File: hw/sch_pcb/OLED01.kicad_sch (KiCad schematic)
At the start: 59 parts, among them J1 HEADER_2x03_PARALLEL, J2 HEADER_2x03_PARALLEL, J3 HEADER_2x01_PARALLEL, J4 HEADER_2x03_PARALLEL, J5 HEADER_1x03, J6 HEADER_2x05_PARALLEL, Q1 BC817-25, Q2 BC817-25, Q3 BC817-25, U1 TLV840, U2 MIC5504-2.5YM5, U3 MAX5026, U5 PCA9306DP

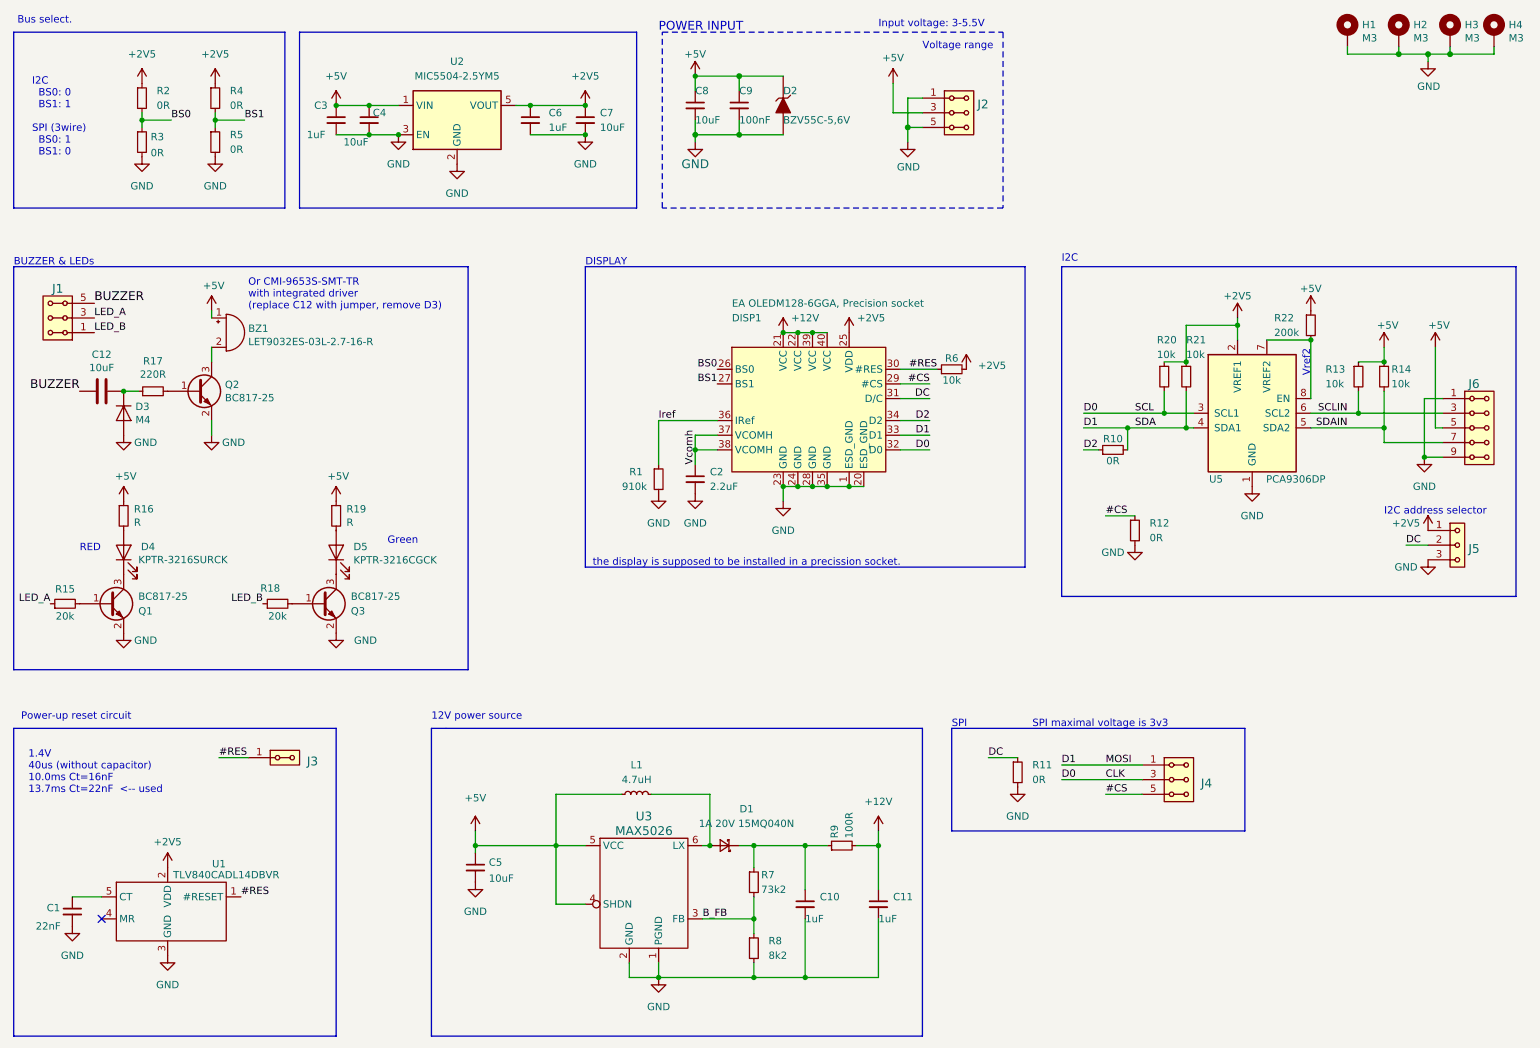
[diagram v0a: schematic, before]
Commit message: solve DRC
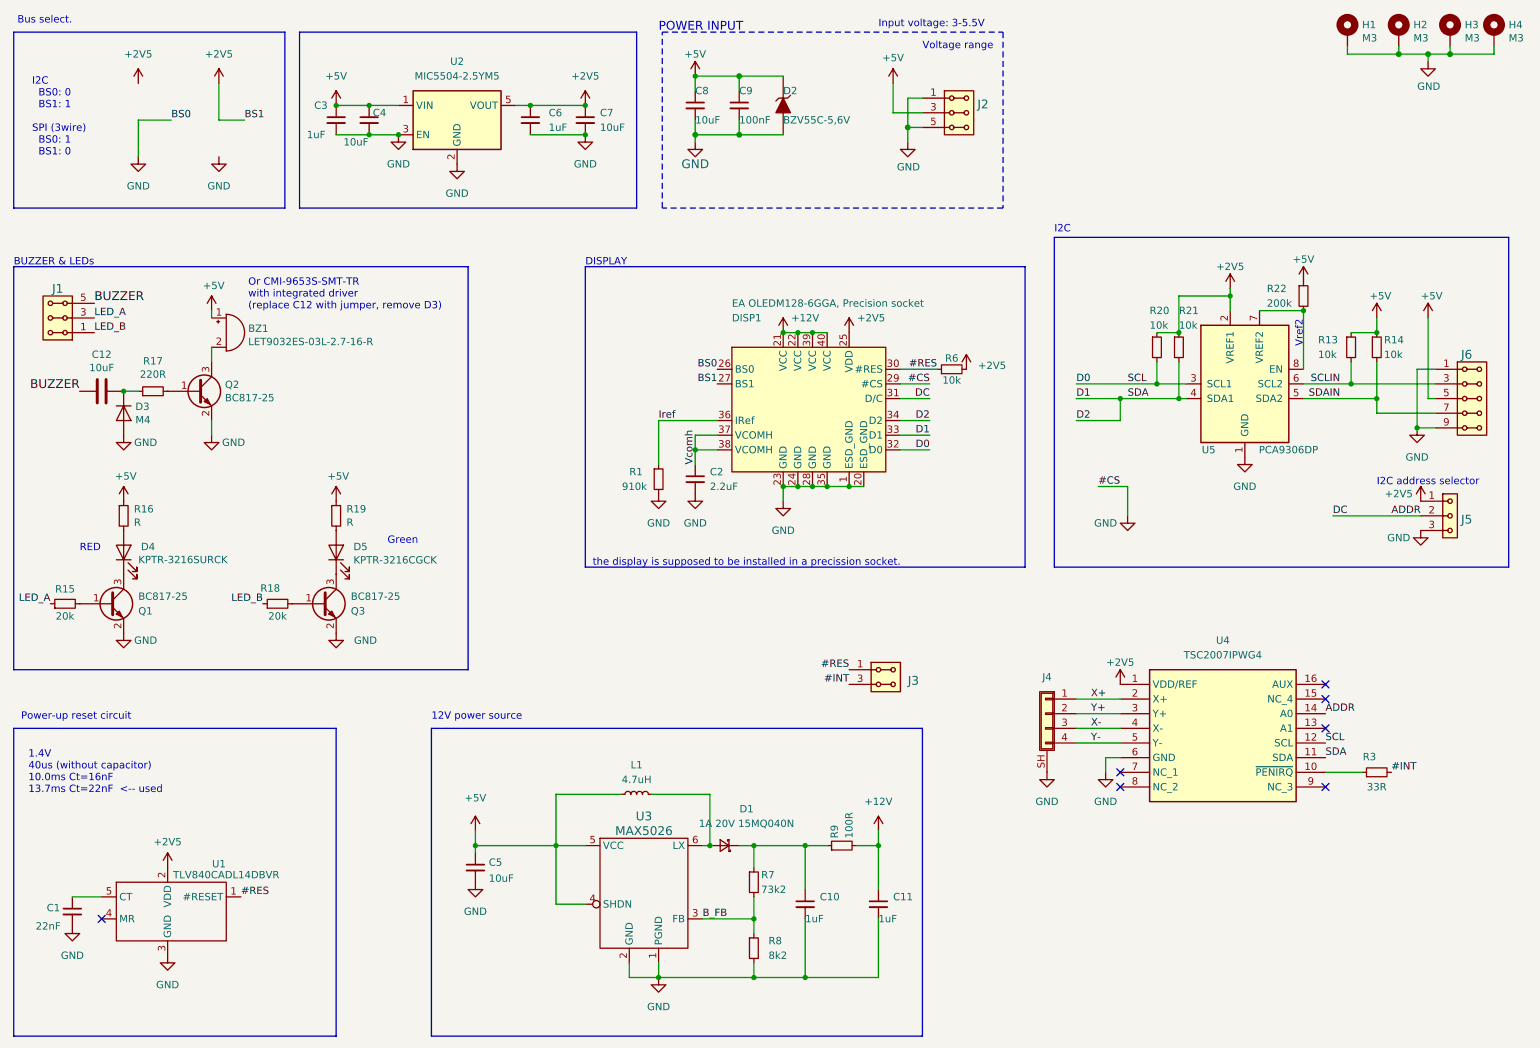
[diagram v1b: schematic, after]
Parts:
- removed J4: HEADER_2x03_PARALLEL, Mlab_Pin_Headers:Straight_2x03, symbol MLAB_HEADER:HEADER_2x03_PARALLEL
- removed R10, R11, R12, R2, R4, R5: 0R, Resistor_SMD:R_0805_2012Metric, symbol Device:R_Small
- added J4: Conn_01x04_Shielded, Mlab_CON:EA_WF100-04S, symbol Connector_Generic_Shielded:Conn_01x04_Shielded
- added U4: TSC2007IPWG4, Mlab_IO:SOP65P640X120-16N, symbol MLAB_IO:TSC2007IPWG4
- J3: footprint Mlab_Pin_Headers:Straight_2x01 -> Mlab_Pin_Headers:Straight_2x02; symbol MLAB_HEADER:HEADER_2x01_PARALLEL -> MLAB_HEADER:HEADER_2x02_PARALLEL
- R3: value 0R -> 33R; UST_ID 5c70984512875079b91f896b -> (none)
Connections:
- net #CS is gone; now on net GND: DISP1.29 (#CS)
- net BS1 is gone; now on net +2V5: DISP1.27 (BS1)
- net D2 is gone; now on net D1: DISP1.34 (D2)
- net +2V5: now also U4.1 (VDD/REF)
- net D1: now also U4.11 (SDA)
- net GND: now also DISP1.26 (BS0), J4.SH (Shield), U4.6 (GND); no longer R3.2
- net BS0: no longer names the net of R3.1
- net BS0: now also U4.10 (~{PENIRQ}); no longer DISP1.26 (BS0)
- net CLK renamed D0
- net D0: now also U4.12 (SCL)
- net DC renamed ADDR
- net ADDR: now also U4.14 (A0)
- new net #INT: J3.3, J3.4, R3.2
- new net X+: J4.1 (Pin_1), U4.2 (X+)
- new net X-: J4.3 (Pin_3), U4.4 (X-)
- new net Y+: J4.2 (Pin_2), U4.3 (Y+)
- new net Y-: J4.4 (Pin_4), U4.5 (Y-)
- no-connect marks 1 -> 7
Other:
- note removed: "SPI"
- note removed: "SPI maximal voltage is 3v3"
- moved on the sheet: J5, J6, R13, R14, R20, R21, R22, U5
